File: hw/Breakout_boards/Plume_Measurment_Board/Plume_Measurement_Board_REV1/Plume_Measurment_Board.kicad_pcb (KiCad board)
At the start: 2 copper layers, 131 x 18.7 mm, 82 parts, among them J2 Conn_01x04, J3 Conn_Coaxial, J4 Conn_01x04, J5 Conn_Coaxial, U10 LMP7721MA/NOPB, U11 LMP2022MA/NOPB, U12 AD7176-2BRUZ, U2 LMP7721MA/NOPB, U3 LMP2022MA/NOPB, U4 AD8475ARMZ, U5 AD8475ARMZ, U6 TPS62153, U7 AD7176-2BRUZ, U8 AD8475ARMZ, U9 AD8475ARMZ

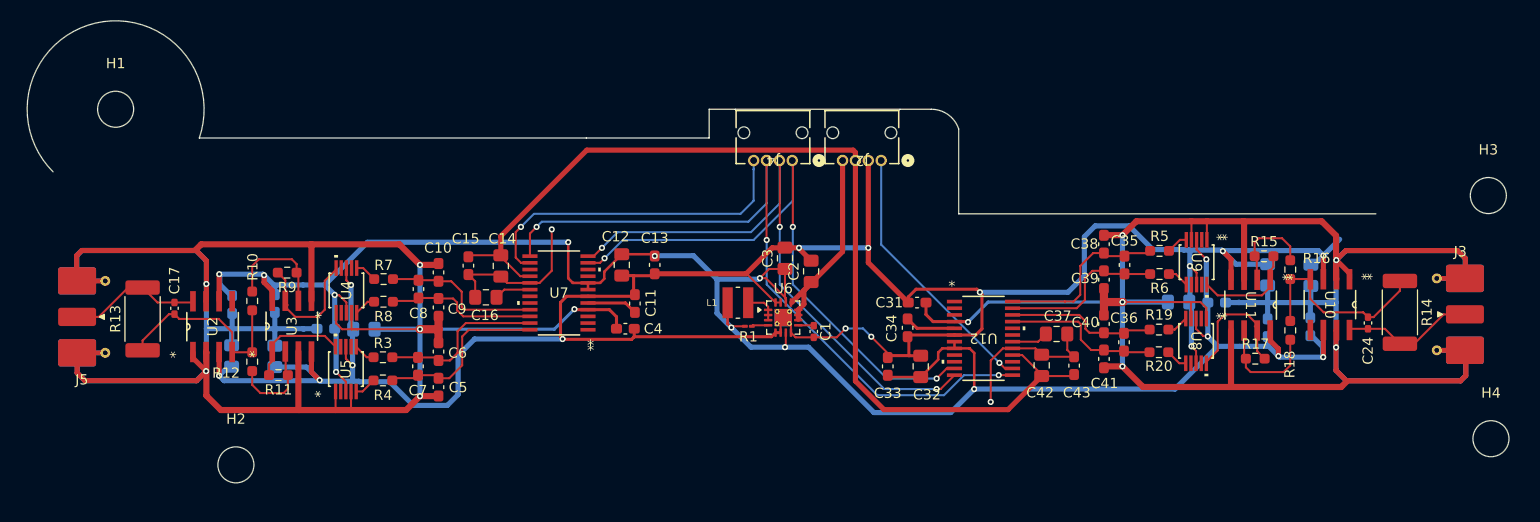
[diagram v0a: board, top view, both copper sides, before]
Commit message: Edge Cuts + Dimension Wor + Awaiting Dimension Approval
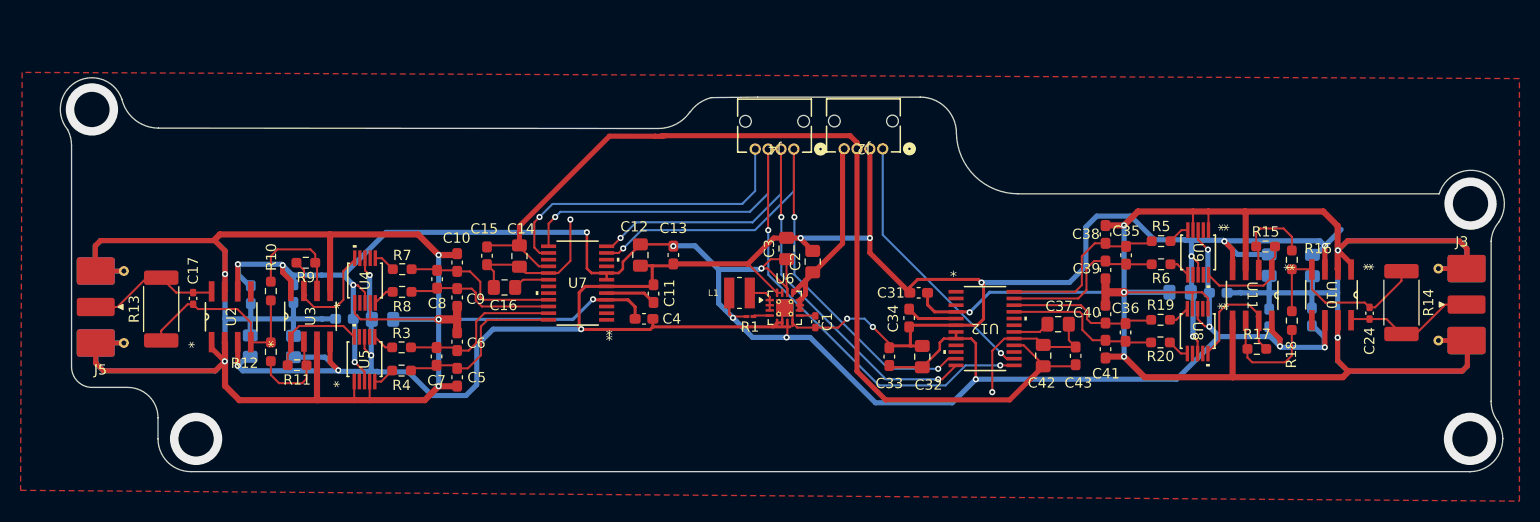
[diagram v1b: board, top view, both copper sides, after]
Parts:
- removed H1, H2, H3, H4: MountingHole, MountingHole:MountingHole_3.5mm
- moved C10 2.05 mm to (117.8, 45.4)
- moved C11 2.05 mm to (136.8, 48.4)
- moved C12 2.05 mm to (135.6, 44.6)
- moved C13 2.05 mm to (138.8, 44.6)
- moved C14 2.05 mm to (123.8, 44.7)
- moved C16 2.05 mm to (122.4, 47.8)
- moved C17 2.05 mm to (92.1, 48.9)
- moved C18 2.05 mm to (110.5, 50.9)
- moved C20 2.05 mm to (101.9, 48.4)
- moved C21 2.05 mm to (97.7, 53.5)
- moved C5 2.05 mm to (117.8, 56.5)
- moved C6 2.05 mm to (117.8, 53.1)
- moved C7 2.05 mm to (115.8, 54.5)
- moved C8 2.05 mm to (115.8, 47.0)
- moved J5 2.05 mm to (82.4, 49.7)
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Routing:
- net /SPI1_MISO: track 58.3 -> 56.6 mm
- net /SPI1_SCK: track 71.8 -> 70.1 mm
- net /SPI1_MOSI: track 58.7 -> 57.0 mm
- net GND: track 283.4 -> 281.7 mm
- net +5V: track 205.3 -> 203.7 mm
- net /PM_CS_1: track 32.4 -> 30.8 mm
- net +3V3: track 96.6 -> 95.3 mm
- net /E-Spray Plume Measurement 2/+2.5V: vias 6 -> 10
- added copper zone on F.Cu, net (none)
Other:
- board size 131 x 18.7 mm -> 140.3 x 38.3 mm
